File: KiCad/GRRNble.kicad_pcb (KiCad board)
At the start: 2 copper layers, 28 x 41 mm, 49 parts, among them J1 JST_SH_06, Q1 DMG3415U, Q2 BSS138, Q3 DMG3415U, SW1 SW_Push, SW2 SW_Push, SW3 SW_Push, U1 R5F100LJAFB, U2 BUZZER, U3 SSD1306, U4 MCP73831, U5 RN4020, U6 NJM2865F33, Y1 32.768k

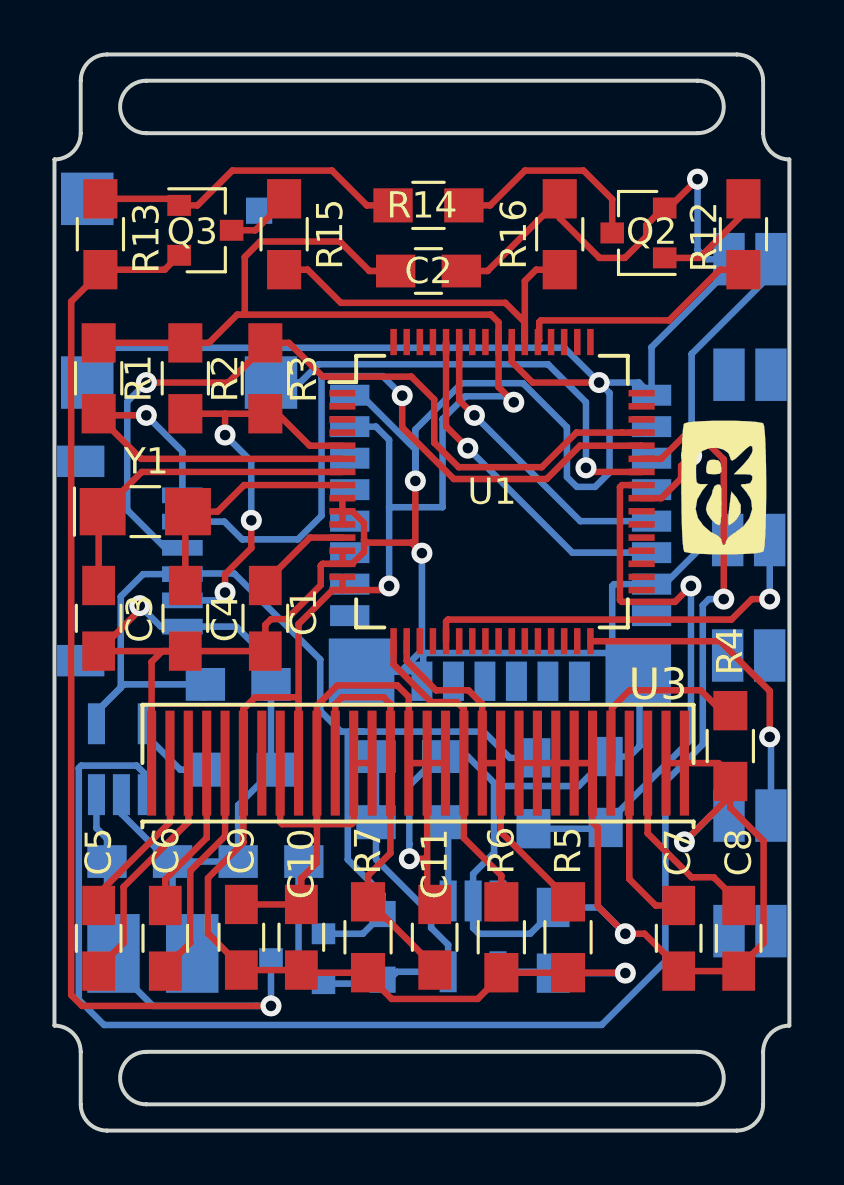
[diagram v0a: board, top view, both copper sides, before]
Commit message: update PCB
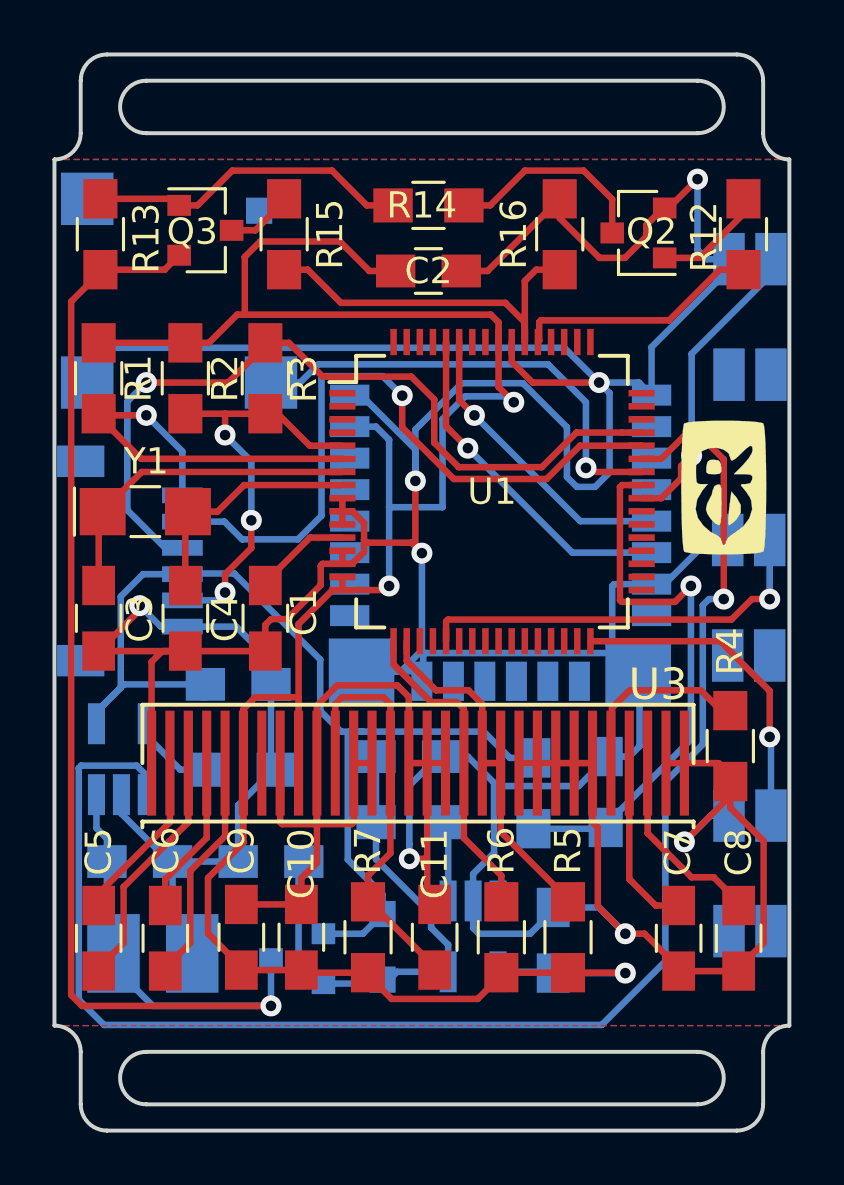
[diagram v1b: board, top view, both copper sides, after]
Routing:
- added copper zone on B.Cu, net GND
- added copper zone on F.Cu, net GND
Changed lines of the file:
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@@
   (via (at 111 94.65) (size 0.8) (drill 0.4) (layers F.Cu B.Cu) (net 38))
   (segment (start 110.17 90.606) (end 110.17 90.982) (width 0.25) (layer F.Cu) (net 38) (status 30))
+  (zone (net 1) (net_name GND) (layer F.Cu) (hatch edge 0.508)
+    (connect_pads (clearance 0.508))
+    (min_thickness 0.254)
+    (fill yes (arc_segments 16) (thermal_gap 0.508) (thermal_bridge_width 0.508))
+    (polygon
+      (pts
+        (xy 95.25 83.65) (xy 123.25 83.65) (xy 123.25 116.65) (xy 95.25 116.65)
+      )
+    )
+  )
+  (zone (net 1) (net_name GND) (layer B.Cu) (hatch edge 0.508)
+    (connect_pads (clearance 0.508))
+    (min_thickness 0.254)
+    (fill yes (arc_segments 16) (thermal_gap 0.508) (thermal_bridge_width 0.508))
+    (polygon
+      (pts
+        (xy 95.25 83.65) (xy 123.25 83.65) (xy 123.25 116.65) (xy 95.25 116.65)
+      )
+    )
+  )
 )
